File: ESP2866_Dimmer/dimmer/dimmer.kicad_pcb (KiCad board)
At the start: 2 copper layers, 84 x 100 mm, 39 parts, among them J1 Screw_Terminal_01x04, J2 Screw_Terminal_01x02, J3 Screw_Terminal_01x04, J4 Conn_01x08, J6 Conn_01x03_Male, J7 Screw_Terminal_01x02, J8 Conn_01x06, J9 Conn_01x16_Female, Q1 2N3904, SW1 Reset, SW2 Menu1, SW3 Menu2, SW4 Menu3, SW5 Menu4, U1 AP1117-33, U2 ESP-12E, U3 AP1117-50, U4 24LC01, U5 PCF8574, U6 PCF8574

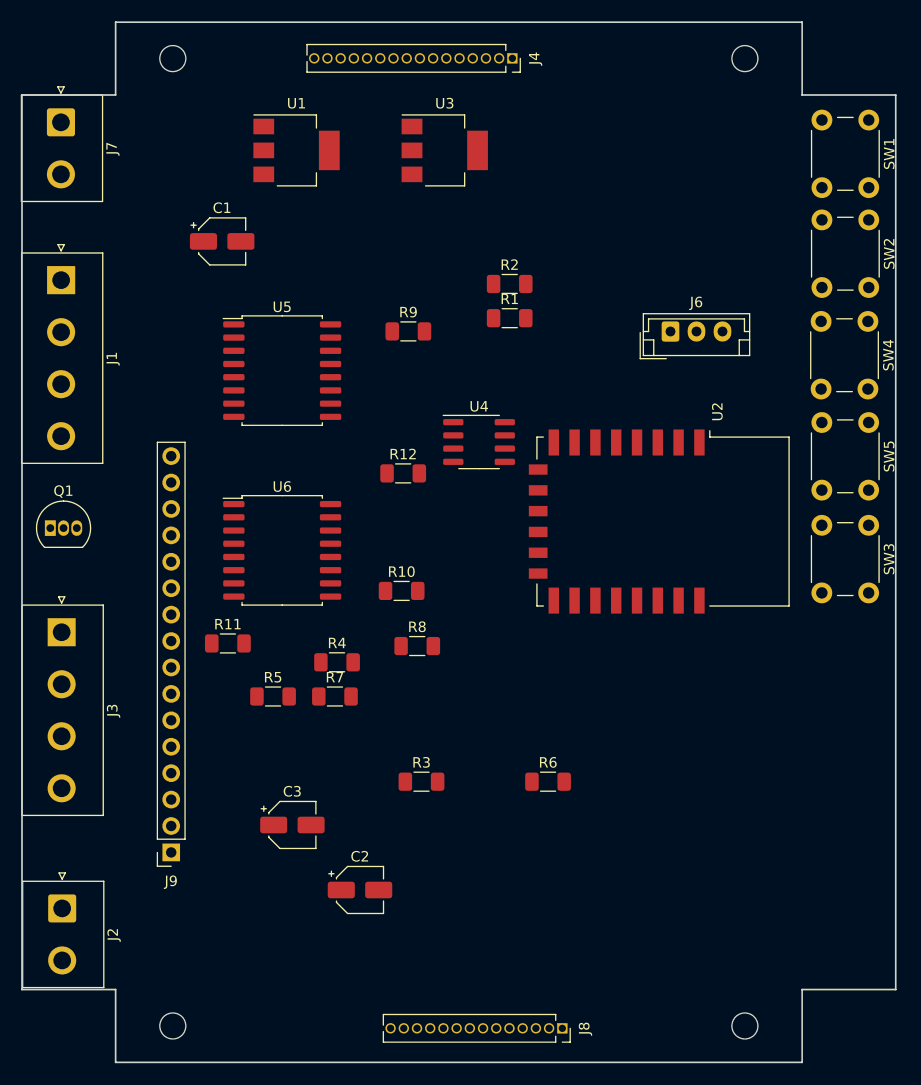
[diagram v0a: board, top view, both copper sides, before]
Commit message: Beta version (fixed)
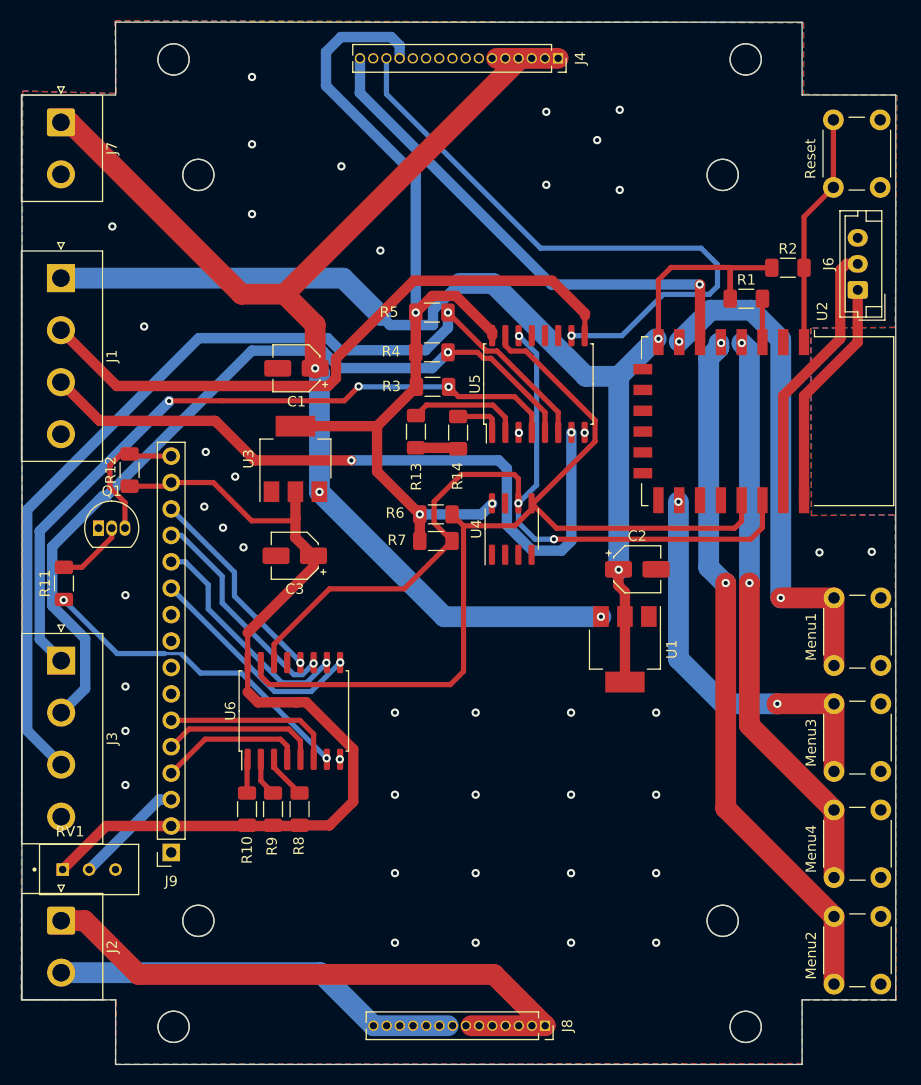
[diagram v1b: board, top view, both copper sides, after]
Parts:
- removed the REF** at (91.3, 150.6)
- removed the REF** at (91.3, 57.6)
- removed the REF** at (36.3, 150.6)
- removed the REF** at (36.3, 57.6)
- added R13: 10k, Resistor_SMD:R_1206_3216Metric_Pad1.30x1.75mm_HandSolder, F.Cu at (59.7, 93.5)
- added R14: 10k, Resistor_SMD:R_1206_3216Metric_Pad1.30x1.75mm_HandSolder, F.Cu at (63.7, 93.6)
- added REF**: MountingHole_3mm, MountingHole:MountingHole_3mm, F.Cu at (38.8, 140.5)
- added REF**: MountingHole_3mm, MountingHole:MountingHole_3mm, F.Cu at (91.4, 57.7)
- added REF**: MountingHole_3mm, MountingHole:MountingHole_3mm, F.Cu at (36.4, 57.7)
- added REF**: MountingHole_3mm, MountingHole:MountingHole_3mm, F.Cu at (89.2, 68.8)
- added REF**: MountingHole_3mm, MountingHole:MountingHole_3mm, F.Cu at (36.4, 150.7)
- added REF**: MountingHole_3mm, MountingHole:MountingHole_3mm, F.Cu at (89.2, 140.5)
- added REF**: MountingHole_3mm, MountingHole:MountingHole_3mm, F.Cu at (91.4, 150.7)
- added REF**: MountingHole_3mm, MountingHole:MountingHole_3mm, F.Cu at (38.8, 68.8)
- added RV1: R_Potentiometer, dimmer:TRIM_3296W-1-203, F.Cu at (28.3, 135.6)
- moved U1 57.4 mm to (79.8, 114.4), turned to -90 degrees
- moved R9 47.7 mm to (45.9, 129.8), turned to 90 degrees
- moved C2 40.8 mm to (81.0, 106.7)
- moved R5 39.9 mm to (61.2, 82.0)
- moved R3 38.0 mm to (61.3, 89.2)
- moved SW3 37.6 mm to (104.4, 140.1)
- moved SW5 37.3 mm to (104.4, 129.9)
- moved SW4 36.8 mm to (104.4, 119.7)
- moved SW2 36.4 mm to (104.4, 109.5)
- moved U3 33.0 mm to (48.1, 96.1), turned to 90 degrees
- moved R4 31.2 mm to (61.2, 85.9)
- moved R6 27.9 mm to (61.6, 101.4)
- moved R2 26.8 mm to (95.4, 77.7)
- moved R12 26.3 mm to (32.1, 97.2), turned to 90 degrees
- moved C3 25.9 mm to (48.0, 105.4), turned to 180 degrees
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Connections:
- J9 pad 15: 5V -> +5V
- J9 pad 2: 5V -> +5V
- R10 pad 1: 5V -> +5V
- R8 pad 1: 5V -> +5V
- R9 pad 1: 5V -> +5V
- U4 pad 8: 5V -> +5V
- U5 pad 1: unconnected-(U5-Pad1) -> Net-(R14-Pad2)
- U5 pad 10: unconnected-(U5-Pad10) -> /LED_ON_RELE
- U5 pad 16: 5V -> +5V
- U5 pad 2: unconnected-(U5-Pad2) -> Net-(R13-Pad2)
- U6 pad 16: 5V -> +5V
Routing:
- net +5V: track 0.00 -> 176.6 mm, vias 0 -> 3
- net +3V3: track 0.00 -> 119.9 mm, vias 0 -> 2
- net +12V: track 0.00 -> 118.6 mm, vias 0 -> 3
- net /DOWN: track 0.00 -> 92.5 mm, vias 0 -> 1
- net /SDA: track 0.00 -> 91.6 mm
- net /SCL: track 0.00 -> 86.4 mm, vias 0 -> 3
- net /UP: track 0.00 -> 79.1 mm, vias 0 -> 1
- net /LIGHT_SENSOR: track 0.00 -> 69.8 mm, vias 0 -> 2
- net /ON_OFF: track 0.00 -> 69.3 mm, vias 0 -> 3
- net /MENU2: track 0.00 -> 67.1 mm, vias 0 -> 2
- net /MOVE_SENSOR: track 0.00 -> 61.4 mm
- net /LED_ON_RELE: track 0.00 -> 60.1 mm, vias 0 -> 1
- net Net-(J2-Pad1): track 0.00 -> 57.8 mm
- net /MENU4: track 0.00 -> 55.1 mm, vias 0 -> 2
- net /PWM_OUT: track 0.00 -> 49.2 mm, vias 0 -> 1
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- added copper zone on B.Cu, net GND
- added copper zone on F.Cu, net GND
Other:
- board size 84 x 100 mm -> 84 x 100.2 mm
